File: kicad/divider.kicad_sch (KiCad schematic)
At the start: 13 parts, among them J40 SPI, Q2 2N3904, Q3 2N3904, U11 TL074, U12 ATtiny24A-P, U13 TL074

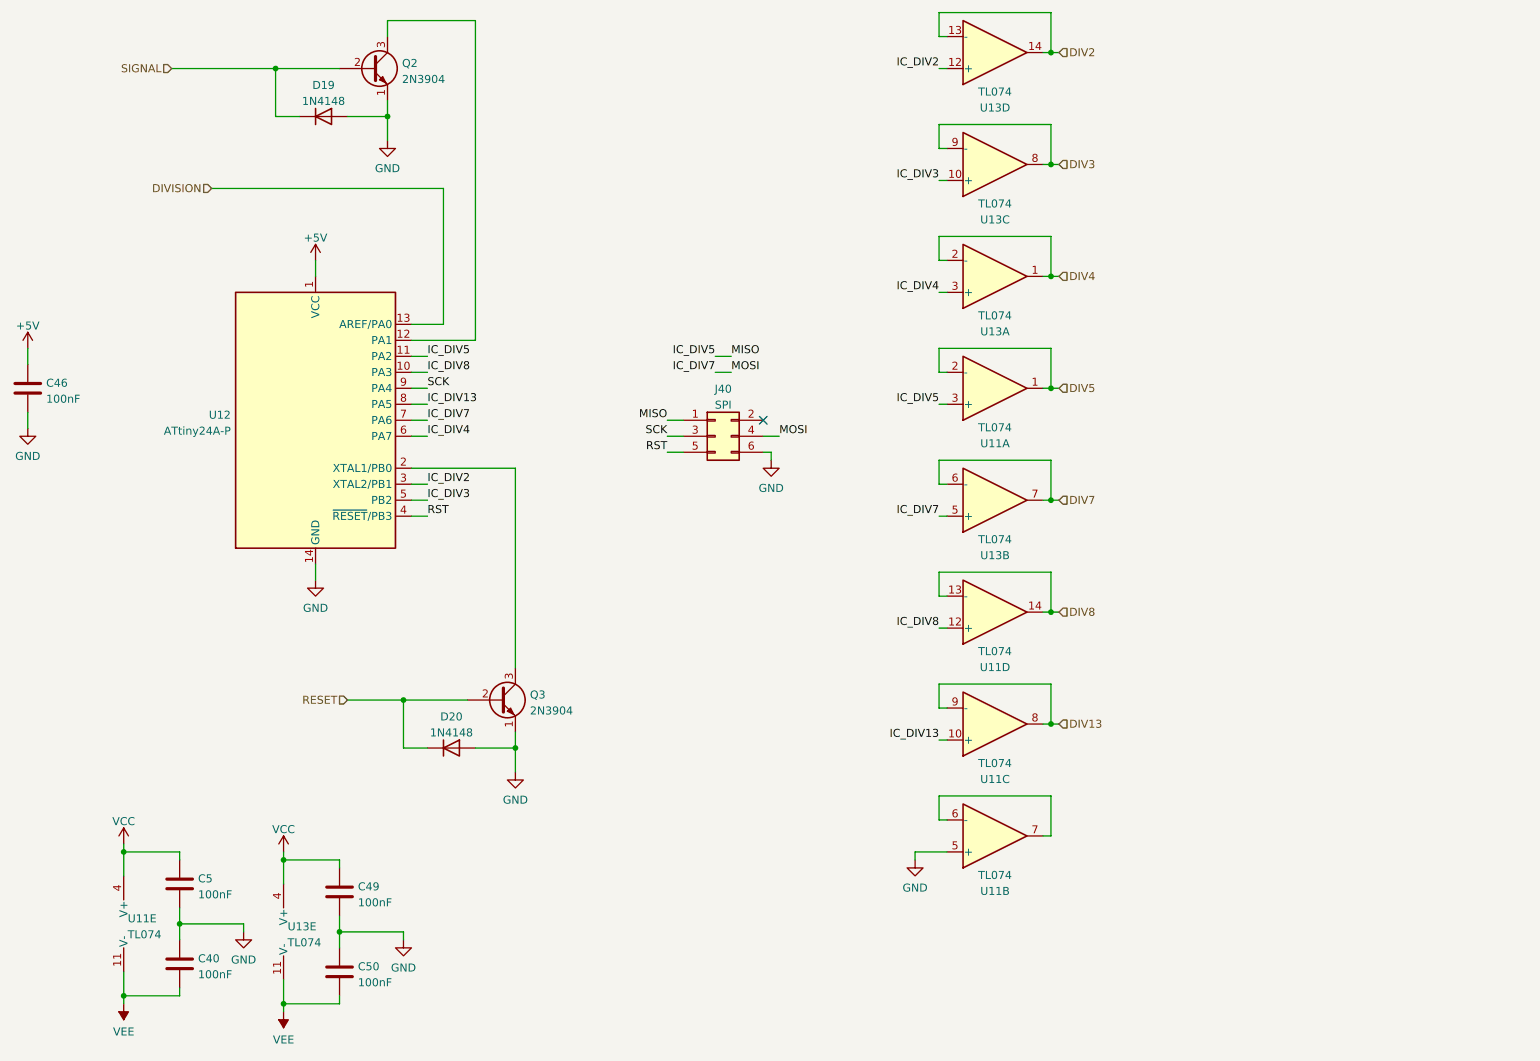
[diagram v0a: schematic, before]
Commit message: Updating layout again
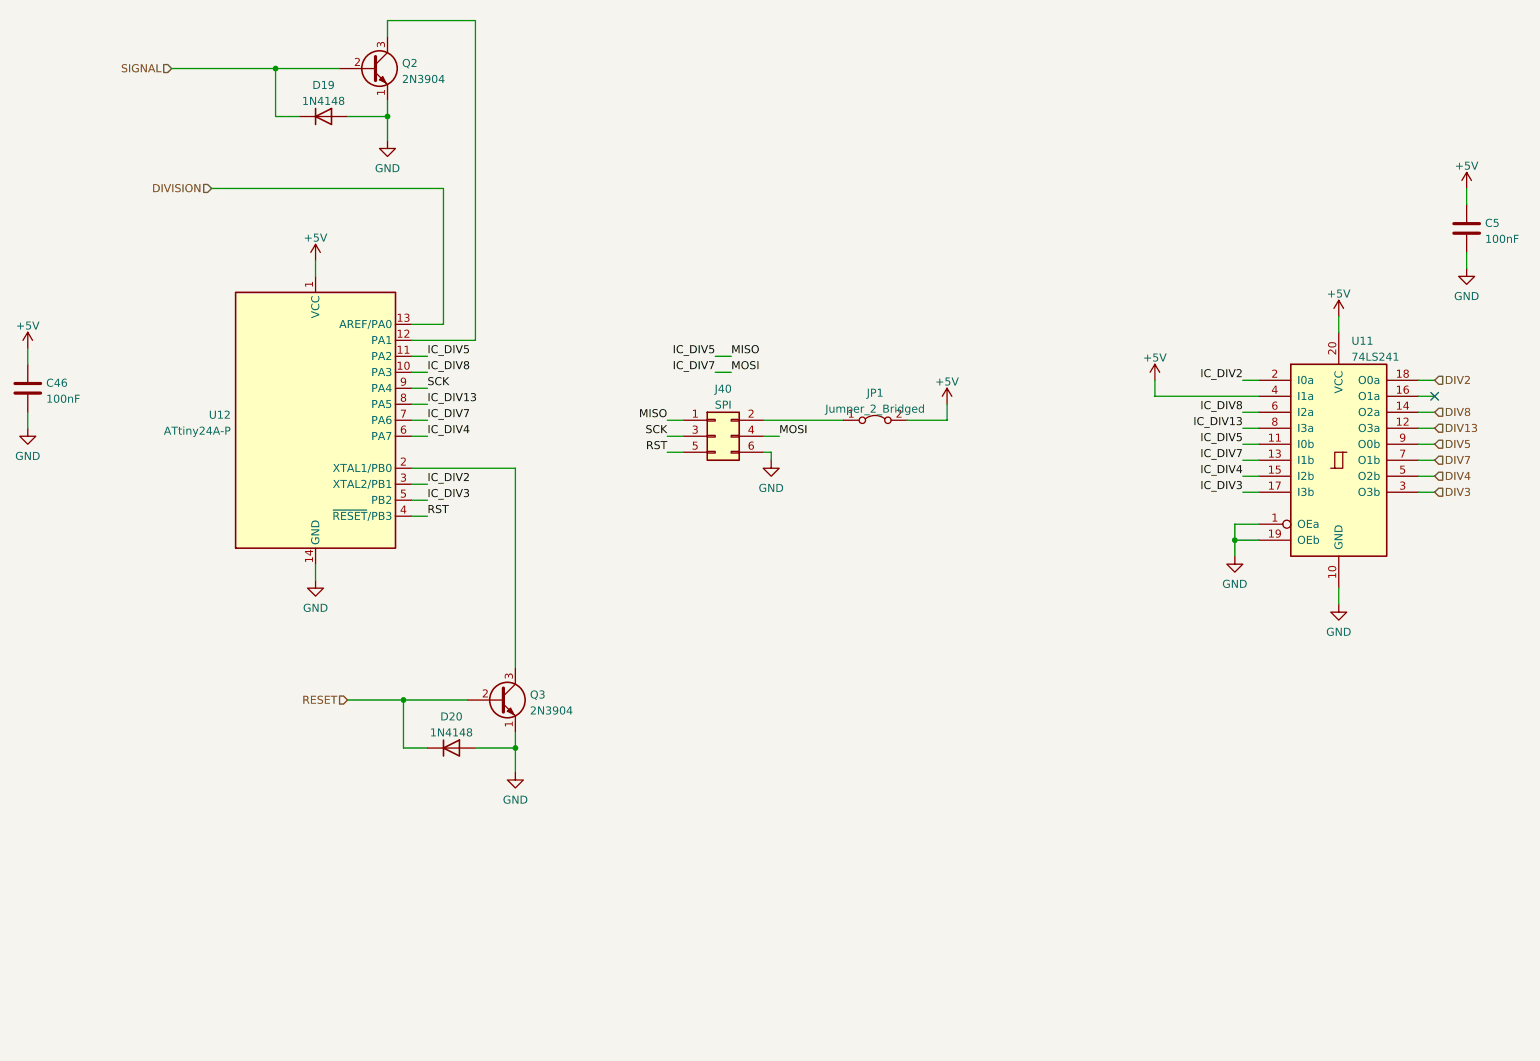
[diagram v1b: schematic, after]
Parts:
- removed C40, C49, C50: 100nF, rumblesan-standard-parts:C_Rect_L7.0mm_W2.5mm_P5.00mm, symbol rumblesan-standard-parts:C
- removed U11, U13: TL074, rumblesan-standard-parts:DIP-14_W7.62mm_Socket, symbol Amplifier_Operational:TL074
- added JP1: Jumper_2_Bridged, Connector_PinHeader_2.54mm:PinHeader_1x02_P2.54mm_Vertical, symbol Jumper:Jumper_2_Bridged
- added U11: 74LS241, Package_DIP:DIP-20_W7.62mm_Socket, symbol 74xx:74LS241
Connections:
- net VCC is gone; now on net +5V: C5.1
- net +5V: now also JP1.2 (B), U11.20 (VCC), U11.4 (I1a)
- net DIV13: now also U11.12 (O3a)
- net DIV2: now also U11.18 (O0a)
- net DIV3: now also U11.3 (O3b)
- net DIV4: now also U11.5 (O2b)
- net DIV5: now also U11.9 (O0b)
- net DIV7: now also U11.7 (O1b)
- net DIV8: now also U11.14 (O2a)
- net GND: now also U11.1 (OEa), U11.10 (GND), U11.19 (OEb)
- net IC_DIV13: now also U11.8 (I3a)
- net IC_DIV2: now also U11.2 (I0a)
- net IC_DIV3: now also U11.17 (I3b)
- net IC_DIV4: now also U11.15 (I2b)
- net IC_DIV5: now also U11.11 (I0b)
- net IC_DIV7: now also U11.13 (I1b)
- net IC_DIV8: now also U11.6 (I2a)
- net at J40.2 (Pin_2): now also JP1.1 (A)
